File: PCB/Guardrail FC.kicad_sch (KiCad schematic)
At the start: 4 parts, among them U1 RP2040, U2 ICM-42688P-HXY, U3 SAM-M8Q-0, U4 SPA06-003

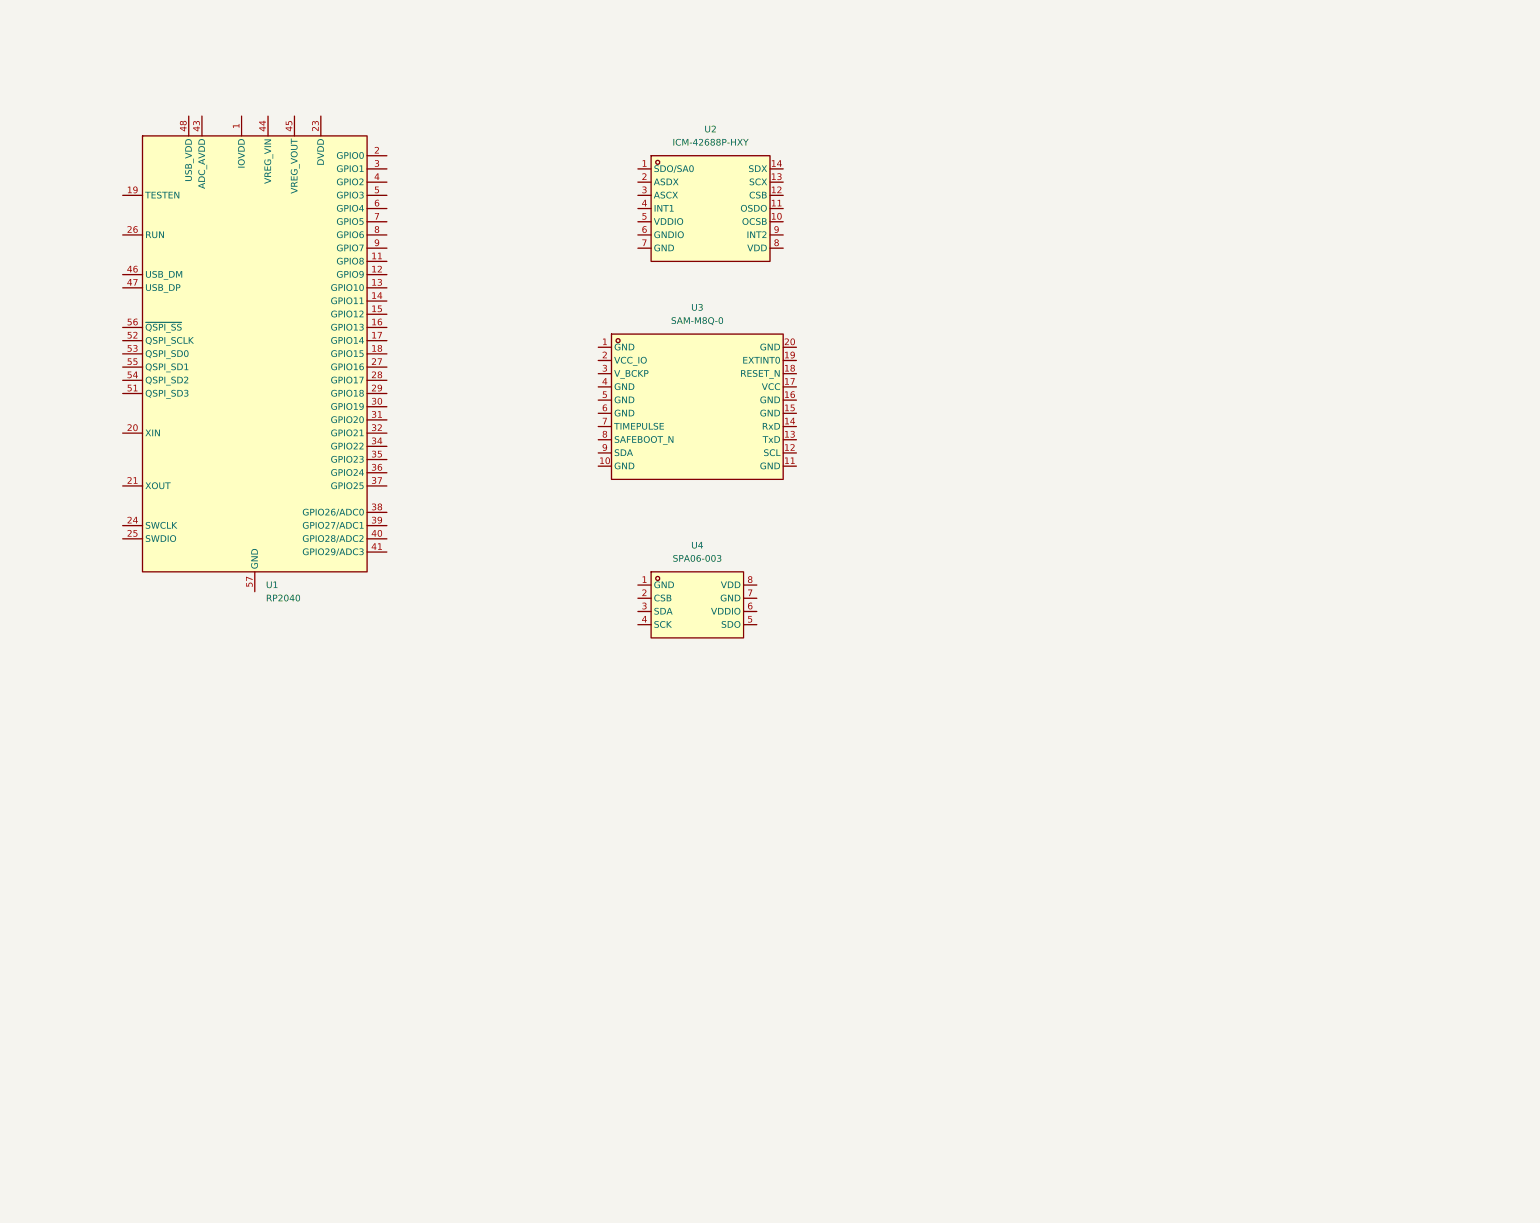
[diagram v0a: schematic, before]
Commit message: PCB Done!
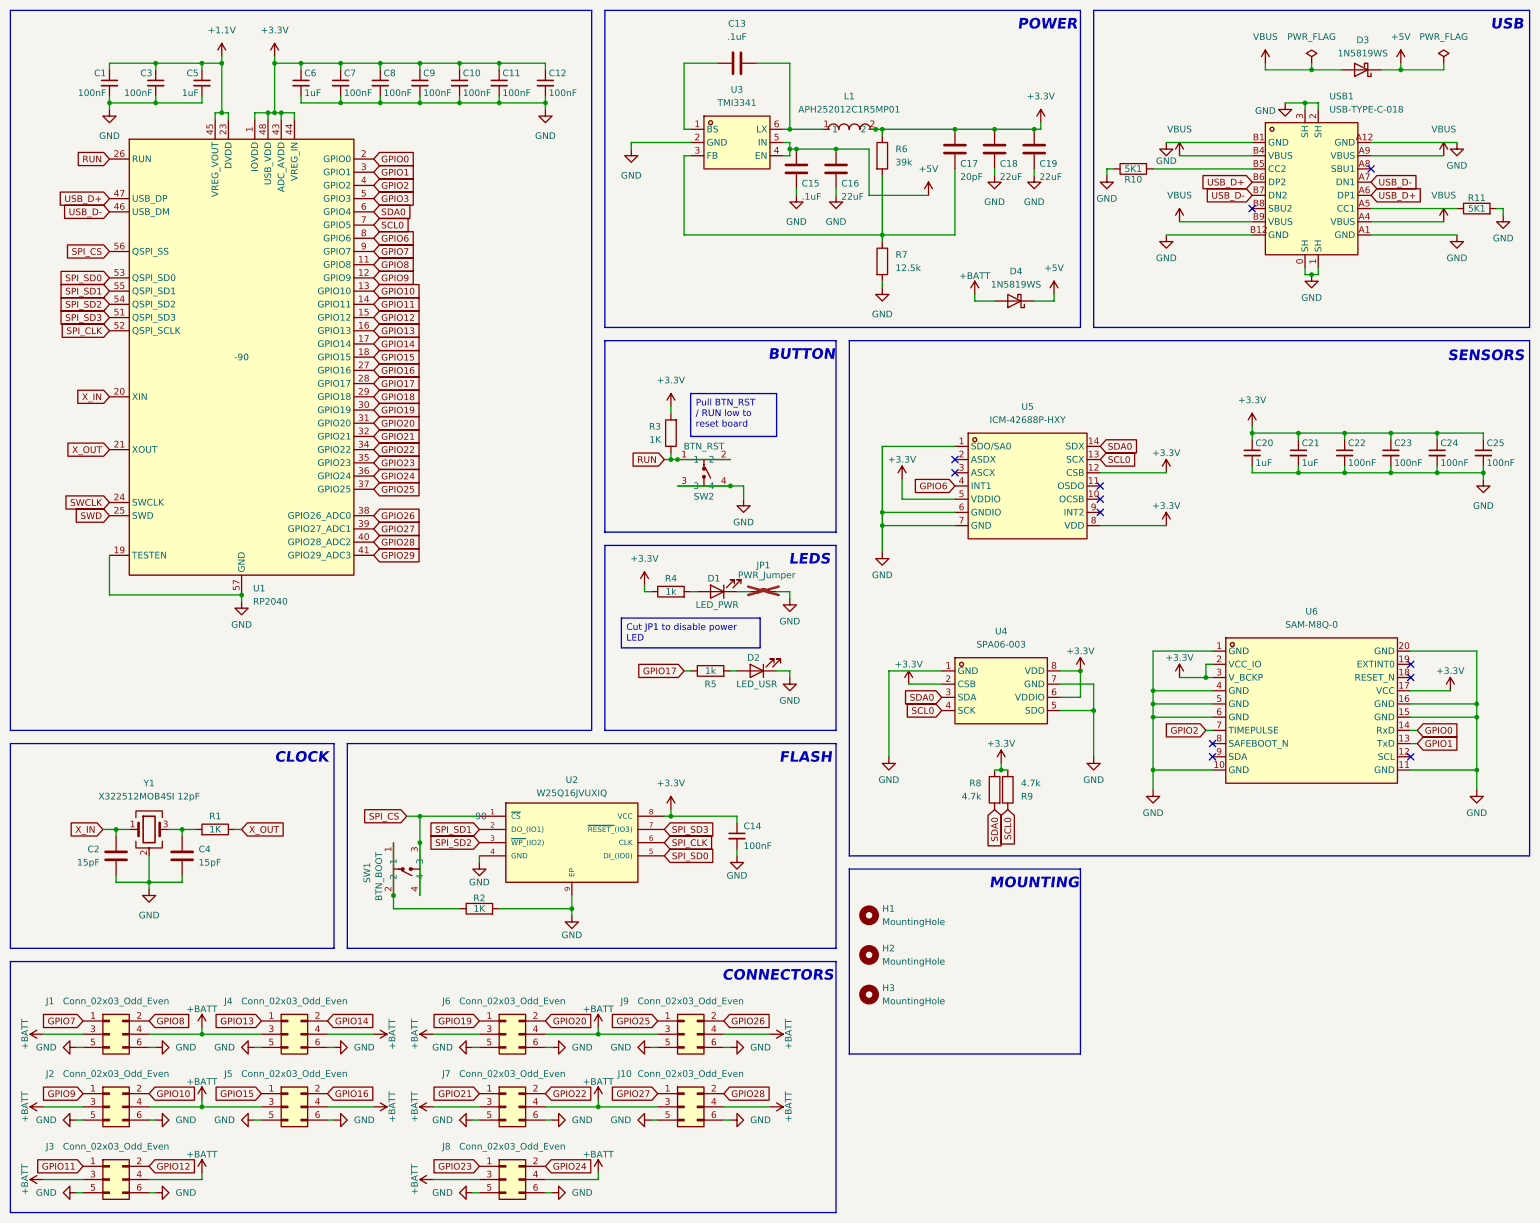
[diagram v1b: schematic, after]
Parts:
- added C1, C10, C11, C12, C14, C22, C23, C24, C25, C3, C7, C8, C9: 100nF, Capacitor_SMD:C_0603_1608Metric_Pad1.08x0.95mm_HandSolder, symbol Device:C_Small
- added C13, C15: .1uF, Capacitor_SMD:C_0603_1608Metric_Pad1.08x0.95mm_HandSolder, symbol Device:C
- added C16, C18, C19: 22uF, Capacitor_SMD:C_0603_1608Metric_Pad1.08x0.95mm_HandSolder, symbol Device:C
- added C17: 20pF, Capacitor_SMD:C_0603_1608Metric_Pad1.08x0.95mm_HandSolder, symbol Device:C
- added C2, C4: 15pF, Capacitor_SMD:C_0603_1608Metric_Pad1.08x0.95mm_HandSolder, symbol Device:C
- added C20, C21, C5, C6: 1uF, Capacitor_SMD:C_0603_1608Metric_Pad1.08x0.95mm_HandSolder, symbol Device:C_Small
- added D1: LED_PWR, LED_SMD:LED_0603_1608Metric, symbol Device:LED
- added D2: LED_USR, LED_SMD:LED_0603_1608Metric, symbol Device:LED
- added D3, D4: 1N5819WS, Diode_SMD:D_SOD-323, symbol Diode:1N5819WS
- added H1, H2, H3: MountingHole, MountingHole:MountingHole_2.2mm_M2_Pad_Via, symbol Mechanical:MountingHole
- added J1, J10, J2, J3, J4, J5, J6, J7, J8, J9: Conn_02x03_Odd_Even, imported_components:HDR-SMD_6P-P2.54-V, symbol Connector_Generic:Conn_02x03_Odd_Even
- added JP1: PWR_Jumper, Jumper:SolderJumper-2_P1.3mm_Bridged2Bar_RoundedPad1.0x1.5mm, symbol Jumper:Jumper_2_Small_Bridged
- added L1: APH252012C1R5MP01, easyeda2kicad:IND-SMD_APH252012C3R3MP01, symbol easyeda2kicad:APH252012C1R5MP01
- added R1, R2, R3: 1K, Resistor_SMD:R_0603_1608Metric_Pad0.98x0.95mm_HandSolder, symbol Device:R
- added R10, R11: 5K1, Resistor_SMD:R_0603_1608Metric_Pad0.98x0.95mm_HandSolder, symbol Device:R
- added R4, R5: 1k, Resistor_SMD:R_0603_1608Metric_Pad0.98x0.95mm_HandSolder, symbol Device:R
- added R6: 39k, Resistor_SMD:R_0603_1608Metric_Pad0.98x0.95mm_HandSolder, symbol Device:R
- added R7: 12.5k, Resistor_SMD:R_0603_1608Metric_Pad0.98x0.95mm_HandSolder, symbol Device:R
- added R8, R9: 4.7k, Resistor_SMD:R_0603_1608Metric_Pad0.98x0.95mm_HandSolder, symbol Device:R
- added SW1: BTN_BOOT, imported_lcsc:SW-SMD_4P-L5.2-W5.2-P5.80-LS6.4, symbol imported_lcsc:LXW-52X52X2-SMD
- added SW2: BTN_RST, imported_lcsc:SW-SMD_4P-L5.2-W5.2-P5.80-LS6.4, symbol imported_lcsc:LXW-52X52X2-SMD
- added U2: W25Q16JVUXIQ, Package_SON:Winbond_USON-8-1EP_3x2mm_P0.5mm_EP0.2x1.6mm, symbol FlashMemory:W25Q16JVUXIQ
- added U3: TMI3341, imported_lcsc:SOT-23-6_L2.9-W1.6-P0.95-LS2.8-BL, symbol imported_lcsc:TMI3341
- added USB1: USB-TYPE-C-018, imported_lcsc:USB-C_SMD-TYPE-C-31-M-12, symbol imported_lcsc:USB-TYPE-C-018
- added Y1: X322512MOB4SI 12pF, Crystal:Crystal_SMD_3225-4Pin_3.2x2.5mm, symbol Device:Crystal_GND24
- U1: FT Rotation Offset (none) -> -90; LCSC (none) -> C2040; private KLC_S4.2_VREG_VOUT -> (none)
- renumbered U2 to U5, U3 to U6
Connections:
- net GND: now reaches U6.1 (GND)
- net GND: now also U1.19 (TESTEN), U1.57 (GND), U4.1 (GND), U4.5 (SDO), U4.7 (GND), U5.1 (SDO/SA0), U5.6 (GNDIO), U5.7 (GND), U6.10 (GND), U6.11 (GND), U6.15 (GND), U6.16 (GND), U6.20 (GND), U6.4 (GND), U6.5 (GND), U6.6 (GND), C1.2, C10.2, C11.2, C12.2, C14.2, C15.1, C16.1, C18.1, C19.1, C2.1, C20.2, C21.2, C22.2, C23.2, C24.2, C25.2, C3.2, C4.2, C5.2, C6.2, C7.2, C8.2, C9.2, D2.1 (K), J1.5 (Pin_5), J1.6 (Pin_6), J10.5 (Pin_5), J10.6 (Pin_6), J2.5 (Pin_5), J2.6 (Pin_6), J3.5 (Pin_5), J3.6 (Pin_6), J4.5 (Pin_5), J4.6 (Pin_6), J5.5 (Pin_5), J5.6 (Pin_6), J6.5 (Pin_5), J6.6 (Pin_6), J7.5 (Pin_5), J7.6 (Pin_6), J8.5 (Pin_5), J8.6 (Pin_6), J9.5 (Pin_5), J9.6 (Pin_6), JP1.2 (B), R10.1, R11.2, R2.2, R7.2, SW2.3, SW2.4, U2.4 (GND), U2.9 (EP), U3.2 (GND), USB1.0 (SH), USB1.1 (SH), USB1.2 (SH), USB1.3 (SH), USB1.A1 (GND), USB1.A12 (GND), USB1.B1 (GND), USB1.B12 (GND), Y1.2 (G), Y1.4 (G)
- net GPIO1: now reaches U6.13 (TxD)
- net GPIO1: now also U1.3 (GPIO1)
- net GPIO0: now reaches U6.14 (RxD)
- net GPIO0: now also U1.2 (GPIO0)
- net +3.3V: now reaches U6.17 (VCC)
- net +3.3V: now also U1.1 (IOVDD), U1.10 (IOVDD), U1.22 (IOVDD), U1.33 (IOVDD), U1.42 (IOVDD), U1.43 (ADC_AVDD), U1.44 (VREG_IN), U1.48 (USB_VDD), U1.49 (IOVDD), U4.2 (CSB), U4.6 (VDDIO), U4.8 (VDD), U5.12 (CSB), U5.5 (VDDIO), U5.8 (VDD), U6.2 (VCC_IO), U6.3 (V_BCKP), C10.1, C11.1, C12.1, C14.1, C17.2, C18.2, C19.2, C20.1, C21.1, C22.1, C23.1, C24.1, C25.1, C6.1, C7.1, C8.1, C9.1, L1.2, R3.2, R4.1, R6.1, R8.1, R9.2, U2.8 (VCC)
- net GPIO2: now reaches U6.7 (TIMEPULSE)
- net GPIO2: now also U1.4 (GPIO2)
- net SCL0: now reaches U5.13 (SCX)
- net SCL0: now also U1.7 (GPIO5), U4.4 (SCK), R9.1
- net SDA0: now reaches U5.14 (SDX)
- net SDA0: now also U1.6 (GPIO4), U4.3 (SDA), R8.2
- net GPIO6: now reaches U5.4 (INT1)
- net GPIO6: now also U1.8 (GPIO6)
- net GPIO8: now reaches U1.11 (GPIO8)
- net GPIO8: now also J1.2 (Pin_2)
- net GPIO9: now reaches U1.12 (GPIO9)
- net GPIO9: now also J2.1 (Pin_1)
- net GPIO10: now reaches U1.13 (GPIO10)
- net GPIO10: now also J2.2 (Pin_2)
- net GPIO11: now reaches U1.14 (GPIO11)
- net GPIO11: now also J3.1 (Pin_1)
- net GPIO12: now reaches U1.15 (GPIO12)
- net GPIO12: now also J3.2 (Pin_2)
- net GPIO13: now reaches U1.16 (GPIO13)
- net GPIO13: now also J4.1 (Pin_1)
- net GPIO14: now reaches U1.17 (GPIO14)
- net GPIO14: now also J4.2 (Pin_2)
- net GPIO15: now reaches U1.18 (GPIO15)
- net GPIO15: now also J5.1 (Pin_1)
- net X_IN: now reaches U1.20 (XIN)
- net X_IN: now also C2.2, Y1.1
- net X_OUT: now reaches U1.21 (XOUT)
- net X_OUT: now also R1.1
- net +1.1V: now reaches U1.23 (DVDD), U1.50 (DVDD)
- net +1.1V: now also U1.45 (VREG_VOUT), C1.1, C3.1, C5.1
- net SWCLK: now reaches U1.24 (SWCLK)
- net SWD: now reaches U1.25 (SWD)
- net RUN: now reaches U1.26 (RUN)
- net RUN: now also R3.1, SW2.1, SW2.2
- net GPIO16: now reaches U1.27 (GPIO16)
- net GPIO16: now also J5.2 (Pin_2)
- net GPIO17: now reaches U1.28 (GPIO17)
- net GPIO17: now also R5.1
- net GPIO18: now reaches U1.29 (GPIO18)
- net GPIO19: now reaches U1.30 (GPIO19)
- net GPIO19: now also J6.1 (Pin_1)
- net GPIO20: now reaches U1.31 (GPIO20)
- net GPIO20: now also J6.2 (Pin_2)
- net GPIO21: now reaches U1.32 (GPIO21)
- net GPIO21: now also J7.1 (Pin_1)
- net GPIO22: now reaches U1.34 (GPIO22)
- net GPIO22: now also J7.2 (Pin_2)
- net GPIO23: now reaches U1.35 (GPIO23)
- net GPIO23: now also J8.1 (Pin_1)
- net GPIO24: now reaches U1.36 (GPIO24)
- net GPIO24: now also J8.2 (Pin_2)
- net GPIO25: now reaches U1.37 (GPIO25)
- net GPIO25: now also J9.1 (Pin_1)
- net GPIO26: now reaches U1.38 (GPIO26_ADC0)
- net GPIO26: now also J9.2 (Pin_2)
- net GPIO27: now reaches U1.39 (GPIO27_ADC1)
- net GPIO27: now also J10.1 (Pin_1)
- net GPIO28: now reaches U1.40 (GPIO28_ADC2)
- net GPIO28: now also J10.2 (Pin_2)
- net GPIO29: now reaches U1.41 (GPIO29_ADC3)
- net USB_D-: now reaches U1.46 (USB_DM)
- net USB_D-: now also USB1.A7 (DN1), USB1.B7 (DN2)
- net USB_D+: now reaches U1.47 (USB_DP)
- net USB_D+: now also USB1.A6 (DP1), USB1.B6 (DP2)
- net GPIO3: now reaches U1.5 (GPIO3)
- net SPI_SD3: now reaches U1.51 (QSPI_SD3)
- net SPI_SD3: now also U2.7 (~{RESET_}(IO3))
- net SPI_CLK: now reaches U1.52 (QSPI_SCLK)
- net SPI_CLK: now also U2.6 (CLK)
- net SPI_SD0: now reaches U1.53 (QSPI_SD0)
- net SPI_SD0: now also U2.5 (DI_(IO0))
- net SPI_SD2: now reaches U1.54 (QSPI_SD2)
- net SPI_SD2: now also U2.3 (~{WP_}(IO2))
- net SPI_SD1: now reaches U1.55 (QSPI_SD1)
- net SPI_SD1: now also U2.2 (DO_(IO1))
- net SPI_CS: now reaches U1.56 (QSPI_SS)
- net SPI_CS: now also SW1.3, SW1.4, U2.1 (~{CS})
- net GPIO7: now reaches U1.9 (GPIO7)
- net GPIO7: now also J1.1 (Pin_1)
- new net: R2.1, SW1.1, SW1.2
- new net: D1.1 (K), JP1.1 (A)
- new net: D1.2 (A), R4.2
- new net: D2.2 (A), R5.2
- new net: C13.1, U3.1 (BS)
- new net: C13.2, L1.1, U3.6 (LX)
- new net: R11.1, USB1.A5 (CC1)
- new net: R10.2, USB1.B5 (CC2)
- new net: C4.1, R1.2, Y1.3
- new net: C17.1, R6.2, R7.1, U3.3 (FB)
- new net +5V: C15.2, C16.2, D3.1 (K), D4.1 (K), U3.4 (EN), U3.5 (IN)
- new net +BATT: D4.2 (A), J1.3 (Pin_3), J1.4 (Pin_4), J10.3 (Pin_3), J10.4 (Pin_4), J2.3 (Pin_3), J2.4 (Pin_4), J3.3 (Pin_3), J3.4 (Pin_4), J4.3 (Pin_3), J4.4 (Pin_4), J5.3 (Pin_3), J5.4 (Pin_4), J6.3 (Pin_3), J6.4 (Pin_4), J7.3 (Pin_3), J7.4 (Pin_4), J8.3 (Pin_3), J8.4 (Pin_4), J9.3 (Pin_3), J9.4 (Pin_4)
- new net VBUS: D3.2 (A), USB1.A4 (VBUS), USB1.A9 (VBUS), USB1.B4 (VBUS), USB1.B9 (VBUS)
- no-connect marks 0 -> 12
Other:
- note added: "BUTTON"
- note added: "CLOCK"
- note added: "CONNECTORS"
- note added: "FLASH"
- note added: "LEDS"
- note added: "MOUNTING"
- note added: "POWER"
- note added: "SENSORS"
- note added: "USB"
- moved on the sheet: U4, U5, U6
